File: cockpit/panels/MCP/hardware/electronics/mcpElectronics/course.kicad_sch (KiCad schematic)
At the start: 12 parts

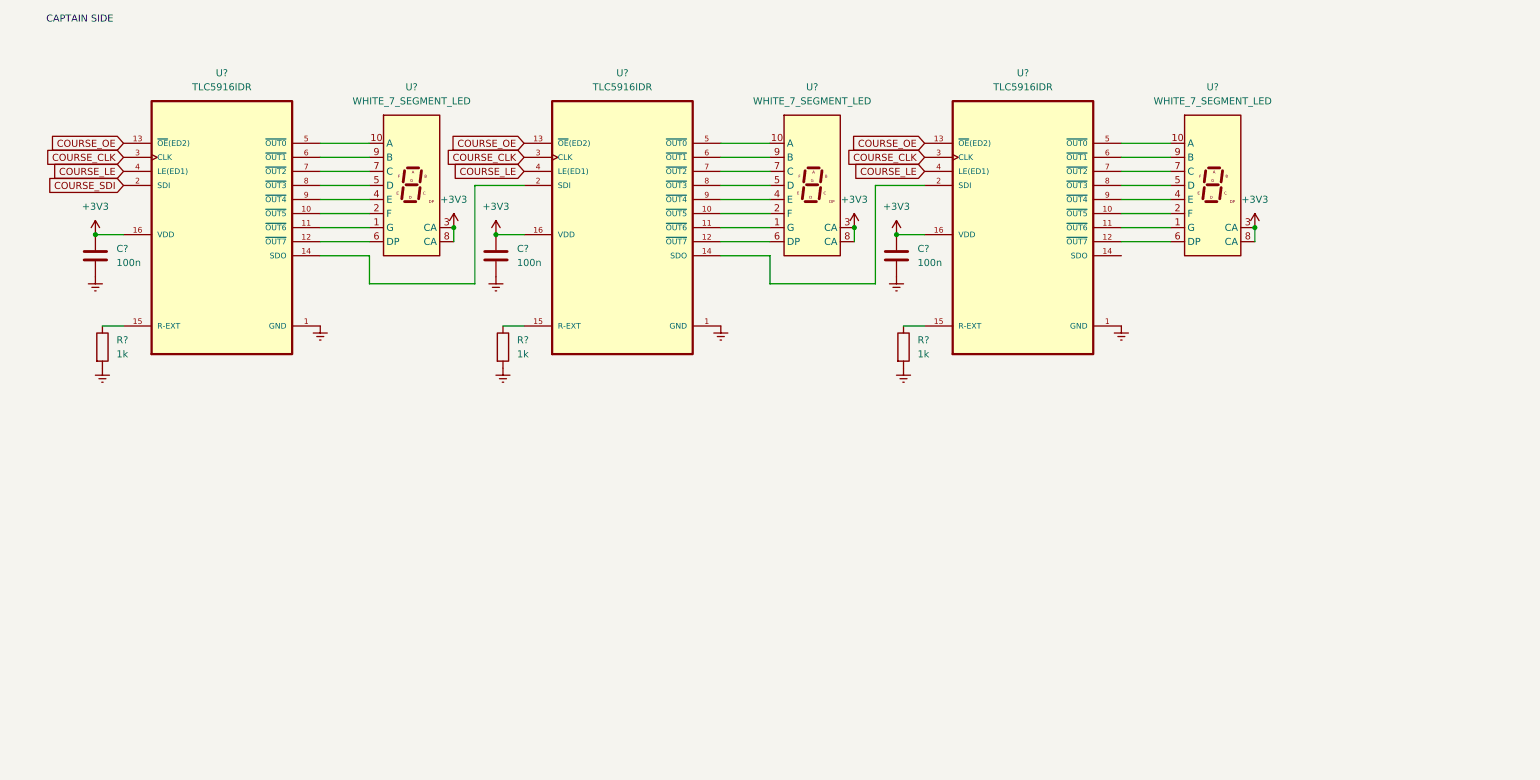
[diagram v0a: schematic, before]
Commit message: add electronics
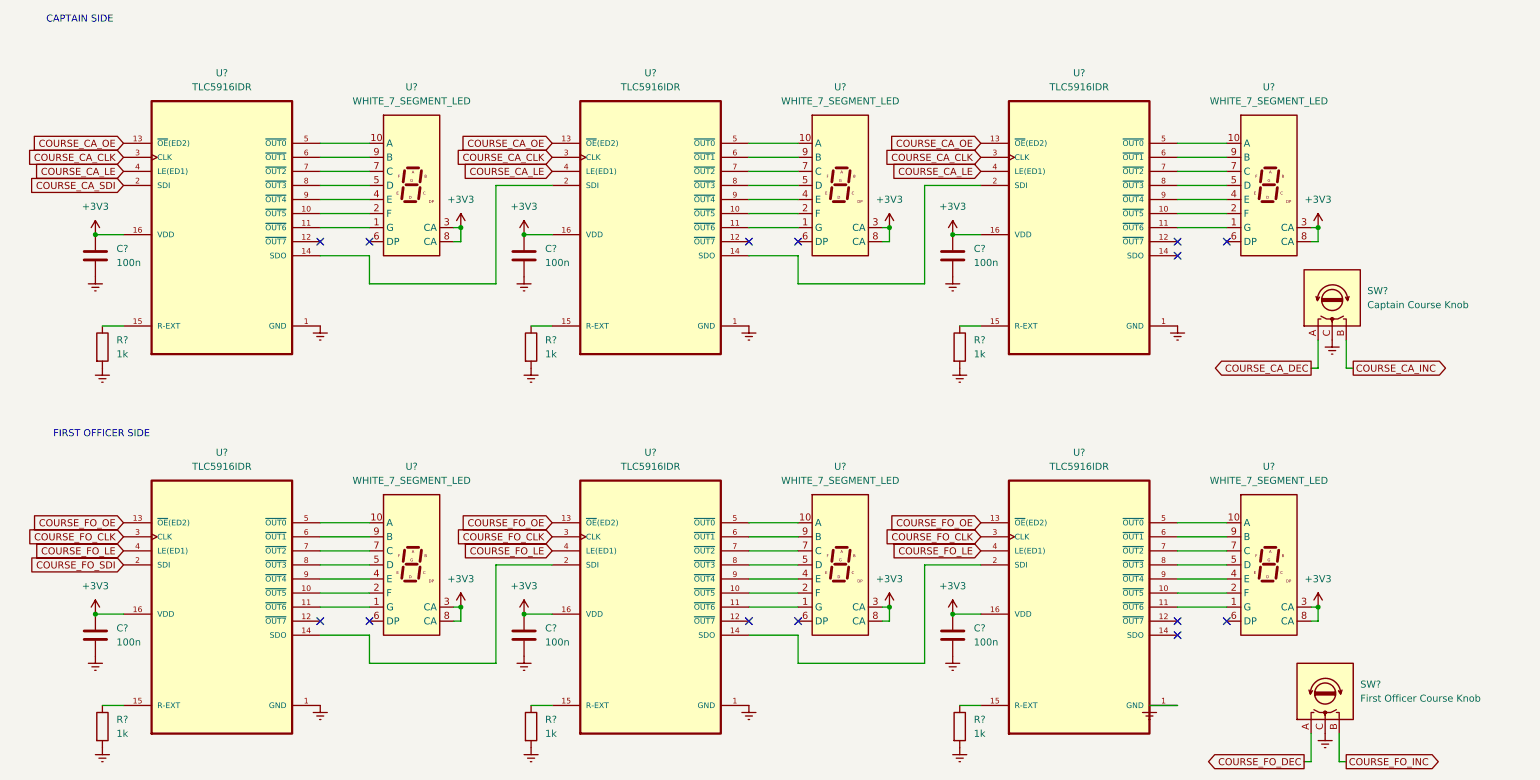
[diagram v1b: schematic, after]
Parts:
- added C? (x3): 100n, symbol Device:C
- added R? (x3): 1k, symbol Device:R
- added SW?: First Officer Course Knob, symbol Device:RotaryEncoder
- added SW?: Captain Course Knob, symbol Device:RotaryEncoder
- added U? (x3): WHITE_7_SEGMENT_LED, Display_7Segment:Sx39-1xxxxx, symbol Display_Character:SA39-11EWA
- added U? (x3): TLC5916IDR, TLC5916IDR:SOIC127P600X175-16N, symbol TLC5916IDR:TLC5916IDR
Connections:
- net +3V3: now also C?.1, C?.1, C?.1, U?.16 (VDD), U?.16 (VDD), U?.16 (VDD), U?.3 (CA), U?.3 (CA), U?.3 (CA), U?.8 (CA), U?.8 (CA), U?.8 (CA)
- net Earth: now also C?.2, C?.2, C?.2, R?.2, R?.2, R?.2, SW?.C, SW?.C, U?.1 (GND), U?.1 (GND), U?.1 (GND)
- net at U?.12 (~{OUT7}): no longer U?.6 (DP) (x2)
- net at U?.6 (DP): no longer U?.12 (~{OUT7})
- net COURSE_CLK renamed COURSE_CA_CLK
- net COURSE_LE renamed COURSE_CA_LE
- net COURSE_OE renamed COURSE_CA_OE
- net COURSE_SDI renamed COURSE_CA_SDI
- new net: U?.1 (G), U?.11 (~{OUT6}) (x3)
- new net: U?.10 (A), U?.5 (~{OUT0}) (x3)
- new net: U?.10 (~{OUT5}), U?.2 (F) (x3)
- new net: U?.4 (E), U?.9 (~{OUT4}) (x3)
- new net: U?.5 (D), U?.8 (~{OUT3}) (x3)
- new net: U?.7 (C), U?.7 (~{OUT2}) (x3)
- new net: U?.6 (~{OUT1}), U?.9 (B) (x3)
- new net: R?.1, U?.15 (R-EXT) (x3)
- new net: U?.14 (SDO), U?.2 (SDI) (x2)
- new net COURSE_CA_DEC: SW?.A
- new net COURSE_CA_INC: SW?.B
- new net COURSE_FO_CLK: U?.3 (CLK), U?.3 (CLK), U?.3 (CLK)
- new net COURSE_FO_DEC: SW?.A
- new net COURSE_FO_INC: SW?.B
- new net COURSE_FO_LE: U?.4 (LE(ED1)), U?.4 (LE(ED1)), U?.4 (LE(ED1))
- new net COURSE_FO_OE: U?.13 (~{OE}(ED2)), U?.13 (~{OE}(ED2)), U?.13 (~{OE}(ED2))
- new net COURSE_FO_SDI: U?.2 (SDI)
- no-connect marks 0 -> 14
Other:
- note added: "FIRST OFFICER SIDE"
- moved on the sheet: C?, R?, U?

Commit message: update
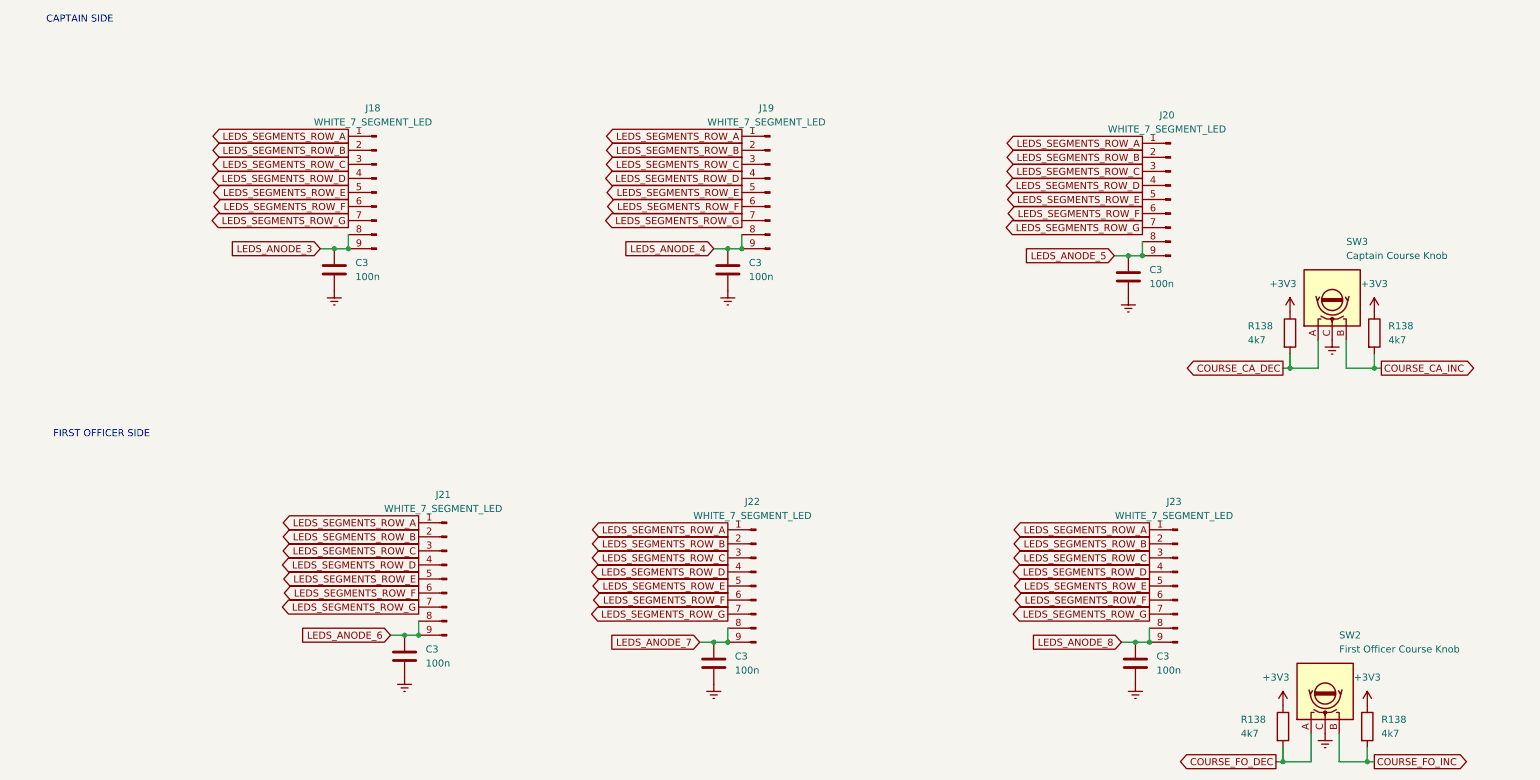
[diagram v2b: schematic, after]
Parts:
- removed C? (x6): 100n, symbol Device:C
- removed R? (x6): 1k, symbol Device:R
- removed U? (x6): TLC5916IDR, TLC5916IDR:SOIC127P600X175-16N, symbol TLC5916IDR:TLC5916IDR
- removed U? (x6): WHITE_7_SEGMENT_LED, Display_7Segment:Sx39-1xxxxx, symbol Display_Character:SA39-11EWA
- added C3 (x6): 100n, Capacitor_SMD:C_0402_1005Metric, symbol Device:C
- added J18, J19, J20, J21, J22, J23: WHITE_7_SEGMENT_LED, Connector_PinHeader_2.54mm:PinHeader_1x09_P2.54mm_Vertical, symbol Connector:Conn_01x09_Pin
- added R138 (x4): 4k7, Resistor_SMD:R_0402_1005Metric, symbol Device:R
- SW2, SW3: renamed from SW?; footprint (none) -> Rotary_Encoder:RotaryEncoder_Bourns_Vertical_PEC12R-3x17F-Nxxxx
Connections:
- net +3V3: now also R138.1, R138.1, R138.1, R138.1
- net COURSE_CA_DEC: now also R138.2
- net COURSE_CA_INC: now also R138.2
- net COURSE_FO_DEC: now also R138.2
- net COURSE_FO_INC: now also R138.2
- net Earth: now also C3.2, C3.2, C3.2, C3.2, C3.2, C3.2
- new net LEDS_ANODE_3: C3.1, J18.8 (Pin_8), J18.9 (Pin_9)
- new net LEDS_ANODE_4: C3.1, J19.8 (Pin_8), J19.9 (Pin_9)
- new net LEDS_ANODE_5: C3.1, J20.8 (Pin_8), J20.9 (Pin_9)
- new net LEDS_ANODE_6: C3.1, J21.8 (Pin_8), J21.9 (Pin_9)
- new net LEDS_ANODE_7: C3.1, J22.8 (Pin_8), J22.9 (Pin_9)
- new net LEDS_ANODE_8: C3.1, J23.8 (Pin_8), J23.9 (Pin_9)
- new net LEDS_SEGMENTS_ROW_A: J18.1 (Pin_1), J19.1 (Pin_1), J20.1 (Pin_1), J21.1 (Pin_1), J22.1 (Pin_1), J23.1 (Pin_1)
- new net LEDS_SEGMENTS_ROW_B: J18.2 (Pin_2), J19.2 (Pin_2), J20.2 (Pin_2), J21.2 (Pin_2), J22.2 (Pin_2), J23.2 (Pin_2)
- new net LEDS_SEGMENTS_ROW_C: J18.3 (Pin_3), J19.3 (Pin_3), J20.3 (Pin_3), J21.3 (Pin_3), J22.3 (Pin_3), J23.3 (Pin_3)
- new net LEDS_SEGMENTS_ROW_D: J18.4 (Pin_4), J19.4 (Pin_4), J20.4 (Pin_4), J21.4 (Pin_4), J22.4 (Pin_4), J23.4 (Pin_4)
- new net LEDS_SEGMENTS_ROW_E: J18.5 (Pin_5), J19.5 (Pin_5), J20.5 (Pin_5), J21.5 (Pin_5), J22.5 (Pin_5), J23.5 (Pin_5)
- new net LEDS_SEGMENTS_ROW_F: J18.6 (Pin_6), J19.6 (Pin_6), J20.6 (Pin_6), J21.6 (Pin_6), J22.6 (Pin_6), J23.6 (Pin_6)
- new net LEDS_SEGMENTS_ROW_G: J18.7 (Pin_7), J19.7 (Pin_7), J20.7 (Pin_7), J21.7 (Pin_7), J22.7 (Pin_7), J23.7 (Pin_7)
- no-connect marks 14 -> 0
